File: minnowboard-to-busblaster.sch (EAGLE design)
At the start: 19 parts, among them J1 CIRCUITCO_MINNOW2_HIGH_SPEED, U1 SN74LV4T125, U2 SN74LV1T125, U3 SN74LV1T125

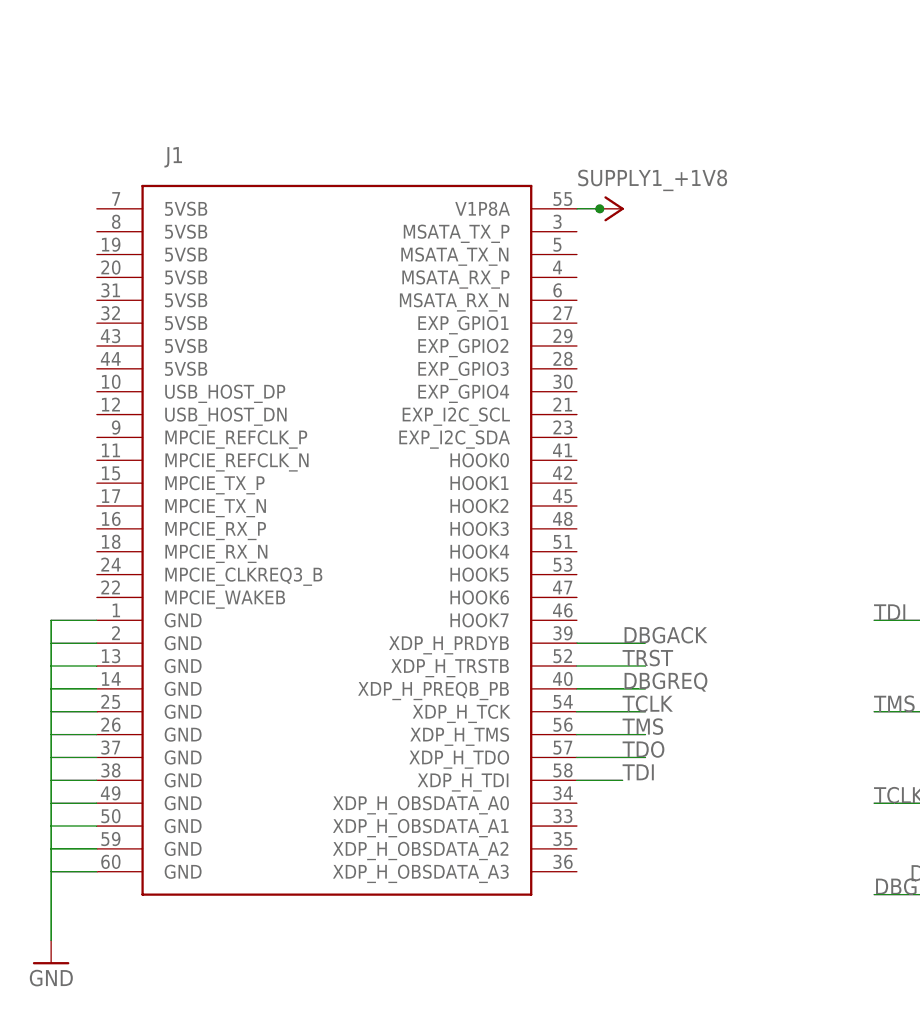
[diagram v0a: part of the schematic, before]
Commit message: all
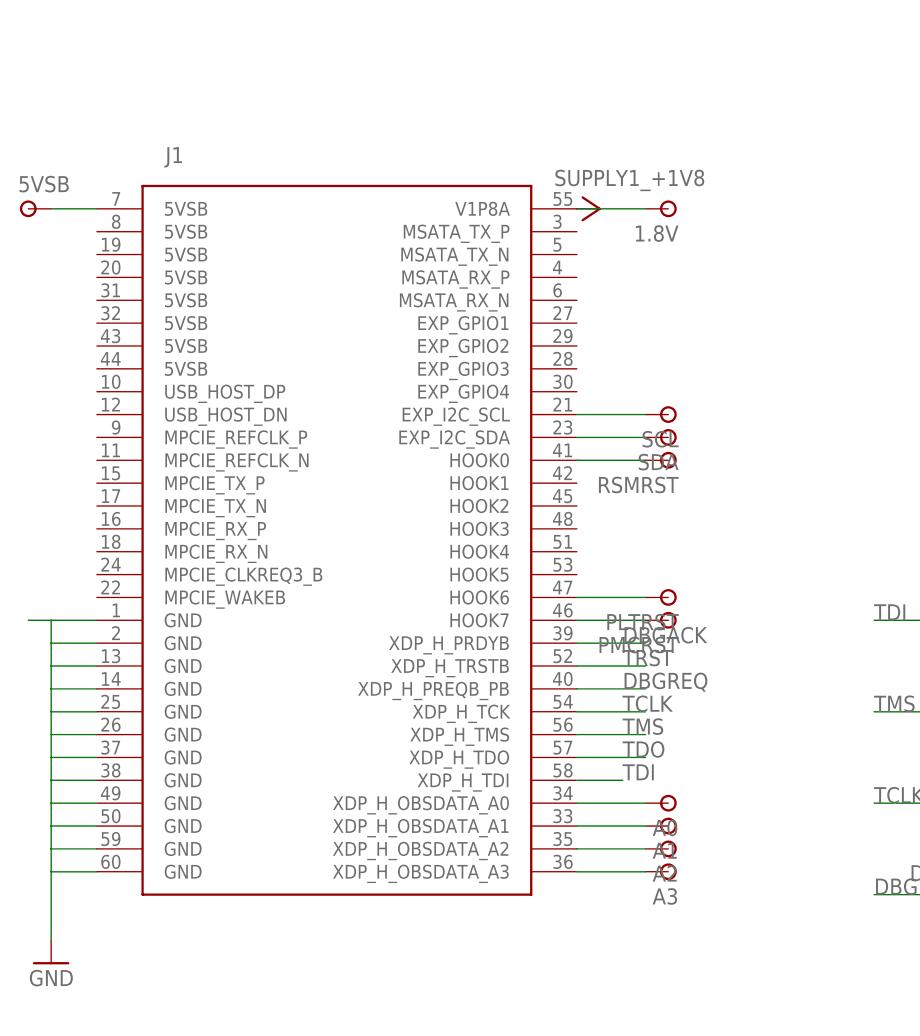
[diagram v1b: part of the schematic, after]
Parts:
- added 1.8V, 5VSB, A0, A1, A2, A3, PLTRST, PMCRST, RSMRST, SCL, SDA: PAD-TESTPOINT, minnowboard:PAD-TESTPOINT
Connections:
- new net N$11: A1.P, J1.XDP_H_OBSDATA_A1
- new net N$13: J1.HOOK0, RSMRST.P
- new net N$14: A3.P, J1.XDP_H_OBSDATA_A3
- new net N$15: J1.EXP_I2C_SCL, SCL.P
- new net N$16: J1.EXP_I2C_SDA, SDA.P
- new net N$7: 5VSB.P, J1.5VSB@1
- new net N$8: A2.P, J1.XDP_H_OBSDATA_A2
- new net N$9: A0.P, J1.XDP_H_OBSDATA_A0
- net +1V8: now also 1.8V.P
- net GND: now also J2.18, J2.20
- net N$23: now also J1.HOOK7, PMCRST.P; no longer J2.18
- net N$24: now also J1.HOOK6, PLTRST.P; no longer J2.20
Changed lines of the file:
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@@
 <setting verticaltext="up"/>
 </settings>
-<grid distance="0.1" unitdist="inch" unit="inch" style="lines" multiple="1" display="yes" altdistance="0.01" altunitdist="inch" altunit="inch"/>
+<grid distance="0.1" unitdist="inch" unit="mm" style="lines" multiple="1" display="yes" altdistance="0.01" altunitdist="inch" altunit="inch"/>
 <layers>
 <layer number="1" name="Top" color="4" fill="1" visible="no" active="no"/>
@@
 <part name="GND7" library="supply1" deviceset="GND" device=""/>
 <part name="GND1" library="supply1" deviceset="GND" device=""/>
+<part name="A0" library="minnowboard" deviceset="PAD-TESTPOINT" device=""/>
+<part name="A1" library="minnowboard" deviceset="PAD-TESTPOINT" device=""/>
+<part name="A2" library="minnowboard" deviceset="PAD-TESTPOINT" device=""/>
+<part name="A3" library="minnowboard" deviceset="PAD-TESTPOINT" device=""/>
+<part name="5VSB" library="minnowboard" deviceset="PAD-TESTPOINT" device=""/>
+<part name="1.8V" library="minnowboard" deviceset="PAD-TESTPOINT" device=""/>
+<part name="SCL" library="minnowboard" deviceset="PAD-TESTPOINT" device=""/>
+<part name="SDA" library="minnowboard" deviceset="PAD-TESTPOINT" device=""/>
+<part name="RSMRST" library="minnowboard" deviceset="PAD-TESTPOINT" device=""/>
+<part name="PLTRST" library="minnowboard" deviceset="PAD-TESTPOINT" device=""/>
+<part name="PMCRST" library="minnowboard" deviceset="PAD-TESTPOINT" device=""/>
 </parts>
 <sheets>
@@
 <instance part="J1" gate="G$1" x="-5.08" y="50.8"/>
 <instance part="J2" gate="A" x="182.88" y="55.88"/>
-<instance part="U$2" gate="G$1" x="25.4" y="88.9" rot="R270"/>
+<instance part="U$2" gate="G$1" x="22.86" y="88.9" rot="R270"/>
 <instance part="U$5" gate="G$1" x="101.6" y="7.62" rot="MR90"/>
 <instance part="TMS1.8" gate="G$1" x="66.04" y="33.02" rot="MR0"/>
@@
 <instance part="GND7" gate="1" x="86.36" y="78.74" rot="MR0"/>
 <instance part="GND1" gate="1" x="-38.1" y="5.08" rot="MR0"/>
+<instance part="A0" gate="P" x="30.48" y="22.86" rot="R180"/>
+<instance part="A1" gate="P" x="30.48" y="20.32" rot="R180"/>
+<instance part="A2" gate="P" x="30.48" y="17.78" rot="R180"/>
+<instance part="A3" gate="P" x="30.48" y="15.24" rot="R180"/>
+<instance part="5VSB" gate="P" x="-40.64" y="88.9"/>
+<instance part="1.8V" gate="P" x="30.48" y="88.9" rot="R180"/>
+<instance part="SCL" gate="P" x="30.48" y="66.04" rot="R180"/>
+<instance part="SDA" gate="P" x="30.48" y="63.5" rot="R180"/>
+<instance part="RSMRST" gate="P" x="30.48" y="60.96" rot="R180"/>
+<instance part="PLTRST" gate="P" x="30.48" y="45.72" rot="R180"/>
+<instance part="PMCRST" gate="P" x="30.48" y="43.18" rot="R180"/>
 </instances>
 <busses>
@@
 <wire x1="-33.02" y1="15.24" x2="-38.1" y2="15.24" width="0.1524" layer="91"/>
 <pinref part="GND1" gate="1" pin="GND"/>
+<wire x1="-38.1" y1="43.18" x2="-40.64" y2="43.18" width="0.1524" layer="91"/>
+</segment>
+<segment>
+<pinref part="J2" gate="A" pin="20"/>
+<wire x1="187.96" y1="43.18" x2="198.12" y2="43.18" width="0.1524" layer="91"/>
+</segment>
+<segment>
+<pinref part="J2" gate="A" pin="18"/>
+<wire x1="187.96" y1="45.72" x2="198.12" y2="45.72" width="0.1524" layer="91"/>
 </segment>
 </net>
@@
 <segment>
 <pinref part="J1" gate="G$1" pin="V1P8A@1"/>
-<wire x1="20.32" y1="88.9" x2="22.86" y2="88.9" width="0.1524" layer="91"/>
 <pinref part="U$2" gate="G$1" pin="+1V8"/>
-<junction x="22.86" y="88.9"/>
+<wire x1="27.94" y1="88.9" x2="20.32" y2="88.9" width="0.1524" layer="91"/>
+<pinref part="1.8V" gate="P" pin="P"/>
 </segment>
 <segment>
@@
 <pinref part="J2" gate="A" pin="16"/>
 <wire x1="187.96" y1="48.26" x2="198.12" y2="48.26" width="0.1524" layer="91"/>
-</segment>
-</net>
-<net name="N$23" class="0">
-<segment>
-<pinref part="J2" gate="A" pin="18"/>
-<wire x1="187.96" y1="45.72" x2="198.12" y2="45.72" width="0.1524" layer="91"/>
-</segment>
-</net>
-<net name="N$24" class="0">
-<segment>
-<pinref part="J2" gate="A" pin="20"/>
-<wire x1="187.96" y1="43.18" x2="198.12" y2="43.18" width="0.1524" layer="91"/>
 </segment>
 </net>
@@
 </segment>
 </net>
+<net name="N$7" class="0">
+<segment>
+<pinref part="J1" gate="G$1" pin="5VSB@1"/>
+<wire x1="-33.02" y1="88.9" x2="-38.1" y2="88.9" width="0.1524" layer="91"/>
+<pinref part="5VSB" gate="P" pin="P"/>
+</segment>
+</net>
+<net name="N$9" class="0">
+<segment>
+<pinref part="J1" gate="G$1" pin="XDP_H_OBSDATA_A0"/>
+<wire x1="27.94" y1="22.86" x2="20.32" y2="22.86" width="0.1524" layer="91"/>
+<pinref part="A0" gate="P" pin="P"/>
+</segment>
+</net>
+<net name="N$11" class="0">
+<segment>
+<pinref part="J1" gate="G$1" pin="XDP_H_OBSDATA_A1"/>
+<wire x1="27.94" y1="20.32" x2="20.32" y2="20.32" width="0.1524" layer="91"/>
+<pinref part="A1" gate="P" pin="P"/>
+</segment>
+</net>
+<net name="N$14" class="0">
+<segment>
+<pinref part="J1" gate="G$1" pin="XDP_H_OBSDATA_A3"/>
+<wire x1="27.94" y1="15.24" x2="20.32" y2="15.24" width="0.1524" layer="91"/>
+<pinref part="A3" gate="P" pin="P"/>
+</segment>
+</net>
+<net name="N$15" class="0">
+<segment>
+<pinref part="J1" gate="G$1" pin="EXP_I2C_SCL"/>
+<wire x1="20.32" y1="66.04" x2="27.94" y2="66.04" width="0.1524" layer="91"/>
+<pinref part="SCL" gate="P" pin="P"/>
+</segment>
+</net>
+<net name="N$16" class="0">
+<segment>
+<pinref part="J1" gate="G$1" pin="EXP_I2C_SDA"/>
+<wire x1="20.32" y1="63.5" x2="27.94" y2="63.5" width="0.1524" layer="91"/>
+<pinref part="SDA" gate="P" pin="P"/>
+</segment>
+</net>
+<net name="N$8" class="0">
+<segment>
+<pinref part="J1" gate="G$1" pin="XDP_H_OBSDATA_A2"/>
+<pinref part="A2" gate="P" pin="P"/>
+<wire x1="20.32" y1="17.78" x2="27.94" y2="17.78" width="0.4064" layer="91"/>
+</segment>
+</net>
+<net name="N$13" class="0">
+<segment>
+<pinref part="J1" gate="G$1" pin="HOOK0"/>
+<wire x1="20.32" y1="60.96" x2="27.94" y2="60.96" width="0.254" layer="91"/>
+<pinref part="RSMRST" gate="P" pin="P"/>
+</segment>
+</net>
+<net name="N$24" class="0">
+<segment>
+<pinref part="J1" gate="G$1" pin="HOOK6"/>
+<wire x1="20.32" y1="45.72" x2="27.94" y2="45.72" width="0.254" layer="91"/>
+<pinref part="PLTRST" gate="P" pin="P"/>
+</segment>
+</net>
+<net name="N$23" class="0">
+<segment>
+<pinref part="J1" gate="G$1" pin="HOOK7"/>
+<wire x1="20.32" y1="43.18" x2="27.94" y2="43.18" width="0.254" layer="91"/>
+<pinref part="PMCRST" gate="P" pin="P"/>
+</segment>
+</net>
